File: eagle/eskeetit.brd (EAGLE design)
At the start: 47 x 28 mm, 46 parts, among them M1 WIRELESS-NRF24L01, U1 GY-521MPU6050, U2 TPS63000DRCR, Y1 20MHz

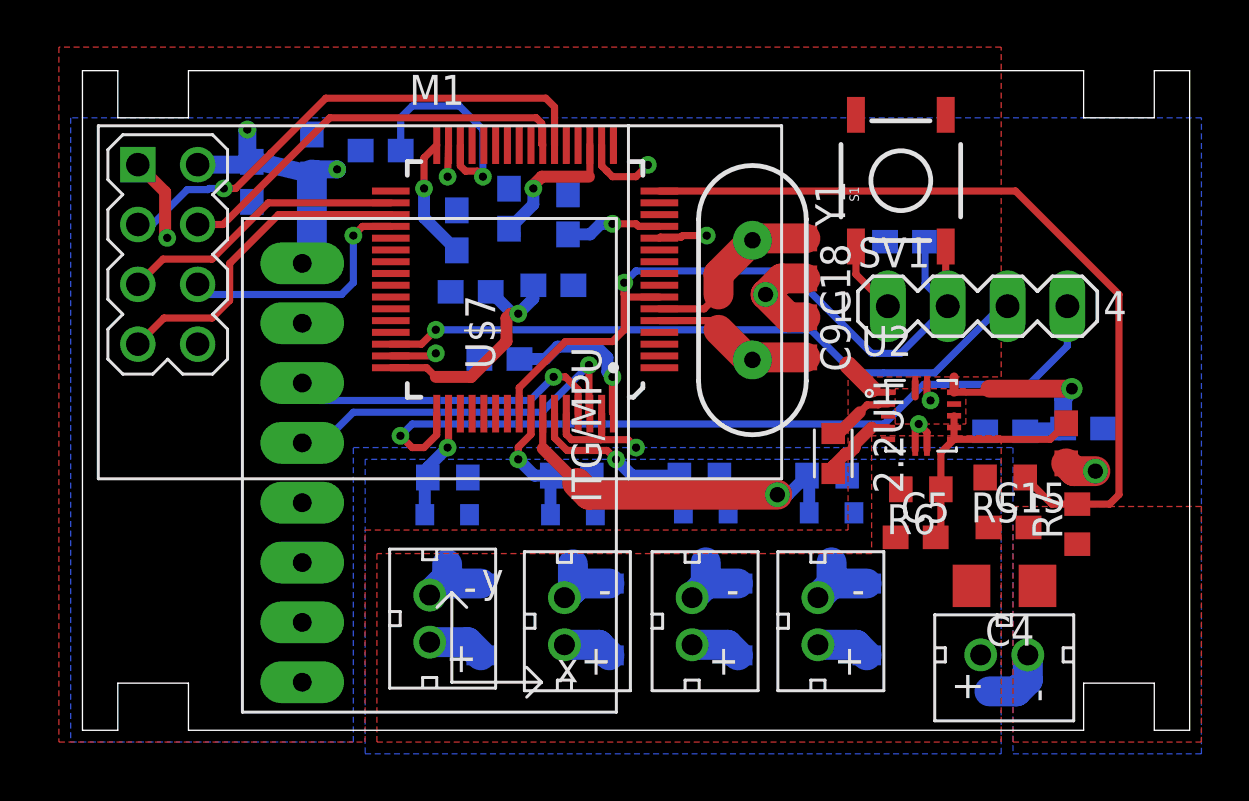
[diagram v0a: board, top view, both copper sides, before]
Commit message: fixed changes in the remote design review
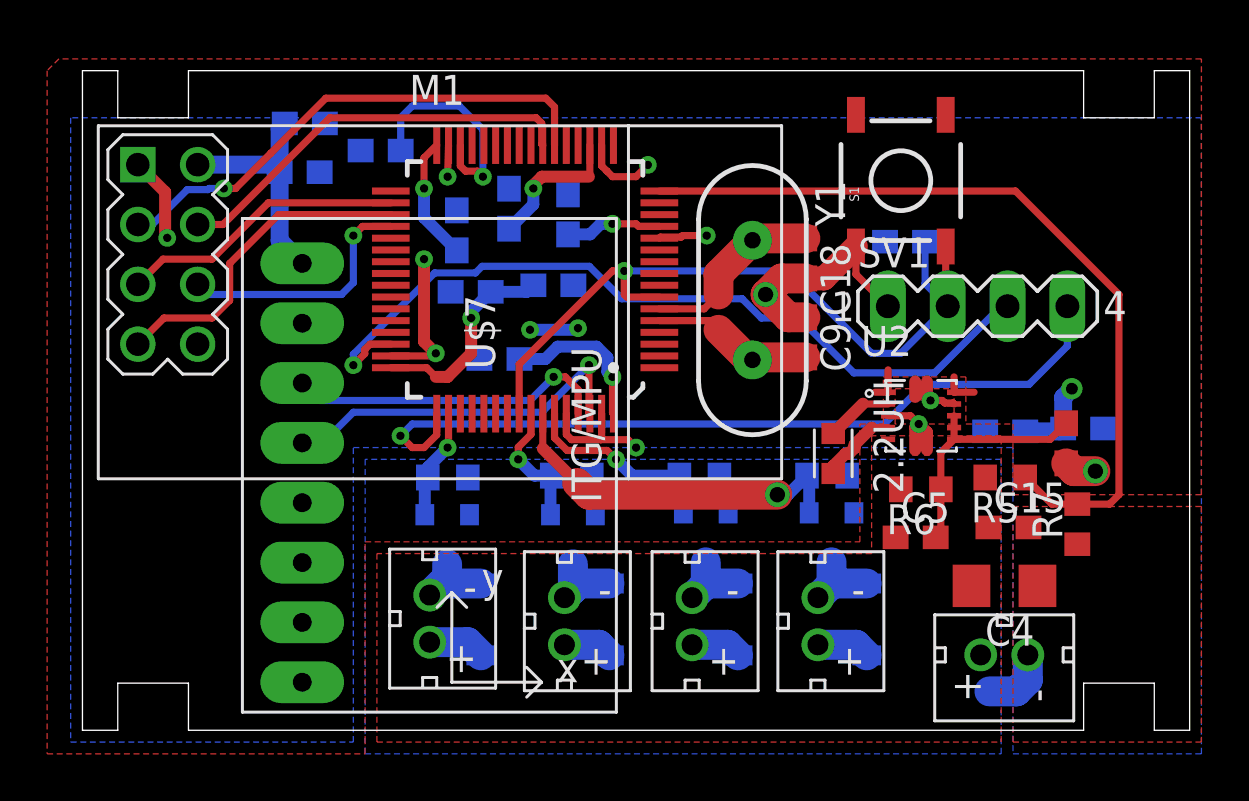
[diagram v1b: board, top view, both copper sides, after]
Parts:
- moved C2 2.07 mm to (9.22, 23.7), turned to 180 degrees
- moved C1 1.35 mm to (9.44, 25.8), turned to 180 degrees
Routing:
- net GND: track 32.8 -> 42.7 mm, vias 10 -> 11
- net SWDIO: track 28.4 -> 34.9 mm
- net 3.3V: track 56.0 -> 49.5 mm
